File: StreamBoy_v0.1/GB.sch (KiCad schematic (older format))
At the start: 43 parts, among them J1 GB-CART, U2 LSF0204PWR, U3 LSF0204PWR

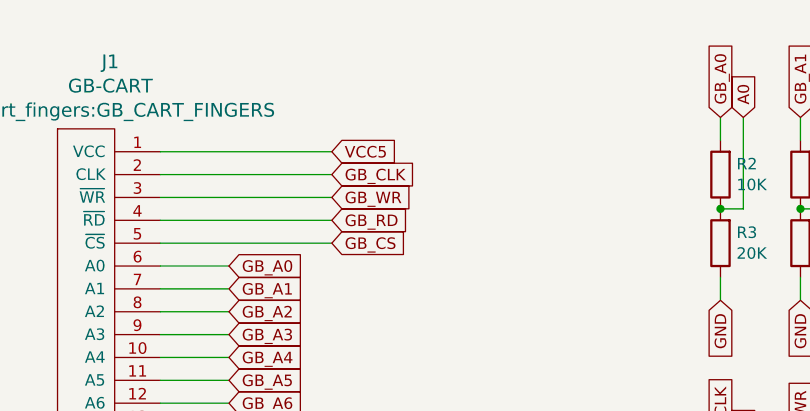
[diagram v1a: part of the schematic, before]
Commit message: Bunch of stuff
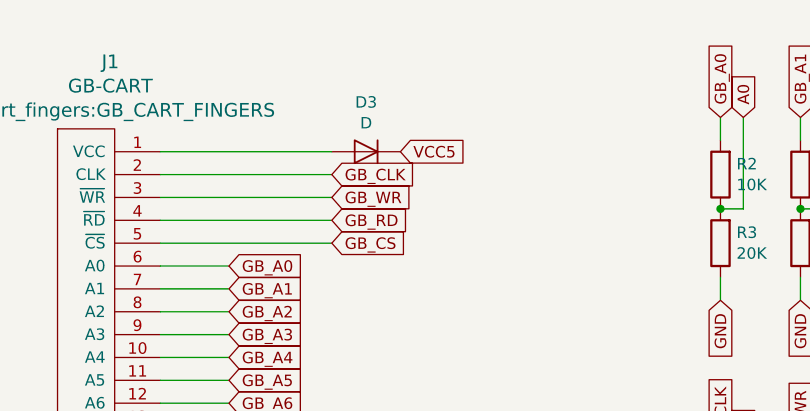
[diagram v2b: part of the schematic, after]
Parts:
- added D3: D, Diode_SMD:D_0805_2012Metric, symbol Device:D
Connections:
- net VCC5: now also D3.1 (K); no longer J1.1 (VCC)
- new net: D3.2 (A), J1.1 (VCC)
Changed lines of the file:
@@
 Text GLabel 3250 1550 2    50   Input ~ 0
 GB_WR
-Text GLabel 3250 1350 2    50   Input ~ 0
-VCC5
 Text GLabel 3250 1450 2    50   Input ~ 0
 GB_CLK
@@
 Text GLabel 3850 6050 0    50   Input ~ 0
 VCC3
+$Comp
+L Device:D D3
+U 1 1 5E09B24F
+P 3400 1350
+F 0 "D3" H 3400 1134 50  0000 C CNN
+F 1 "D" H 3400 1225 50  0000 C CNN
+F 2 "Diode_SMD:D_0805_2012Metric" H 3400 1350 50  0001 C CNN
+F 3 "~" H 3400 1350 50  0001 C CNN
+	1    3400 1350
+	-1   0    0    1
+$EndComp
+Text GLabel 3550 1350 2    50   Input ~ 0
+VCC5
 $EndSCHEMATC

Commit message: Power to the masses
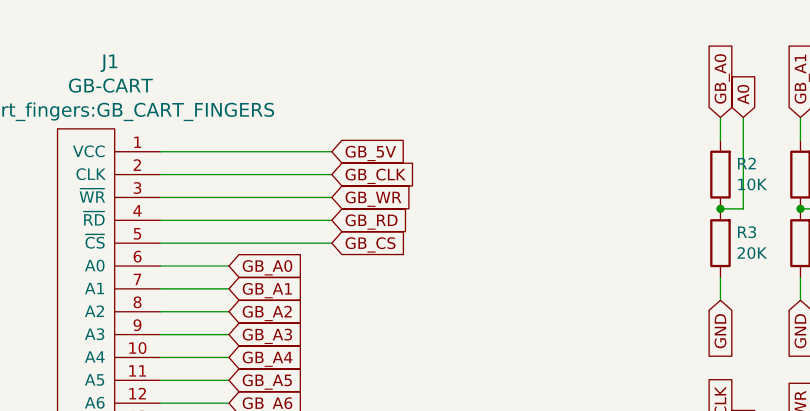
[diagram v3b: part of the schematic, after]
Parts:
- removed D3: D, Diode_SMD:D_0805_2012Metric, symbol Device:D
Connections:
- net GB_5V: now reaches J1.1 (VCC)
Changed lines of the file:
@@
 Text GLabel 3850 6050 0    50   Input ~ 0
 VCC3
-$Comp
-L Device:D D3
-U 1 1 5E09B24F
-P 3400 1350
-F 0 "D3" H 3400 1134 50  0000 C CNN
-F 1 "D" H 3400 1225 50  0000 C CNN
-F 2 "Diode_SMD:D_0805_2012Metric" H 3400 1350 50  0001 C CNN
-F 3 "~" H 3400 1350 50  0001 C CNN
-	1    3400 1350
-	-1   0    0    1
-$EndComp
-Text GLabel 3550 1350 2    50   Input ~ 0
-VCC5
+Text GLabel 3250 1350 2    50   Input ~ 0
+GB_5V
 $EndSCHEMATC

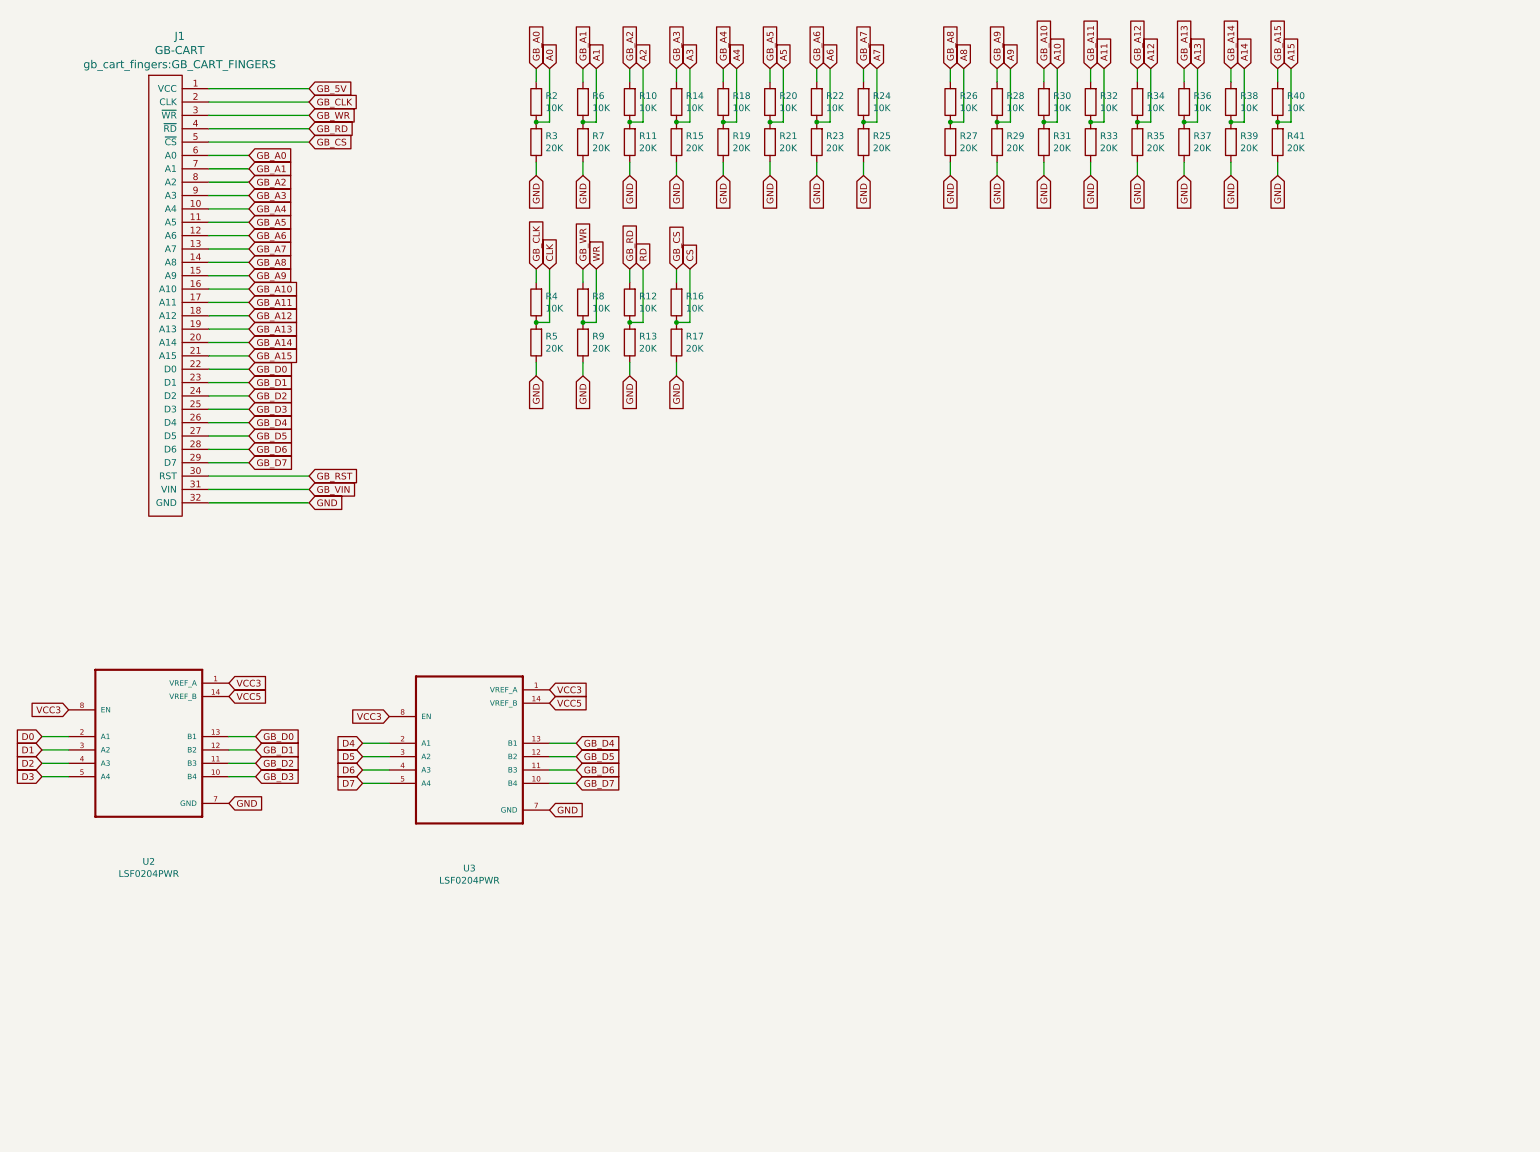
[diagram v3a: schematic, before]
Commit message: Temp
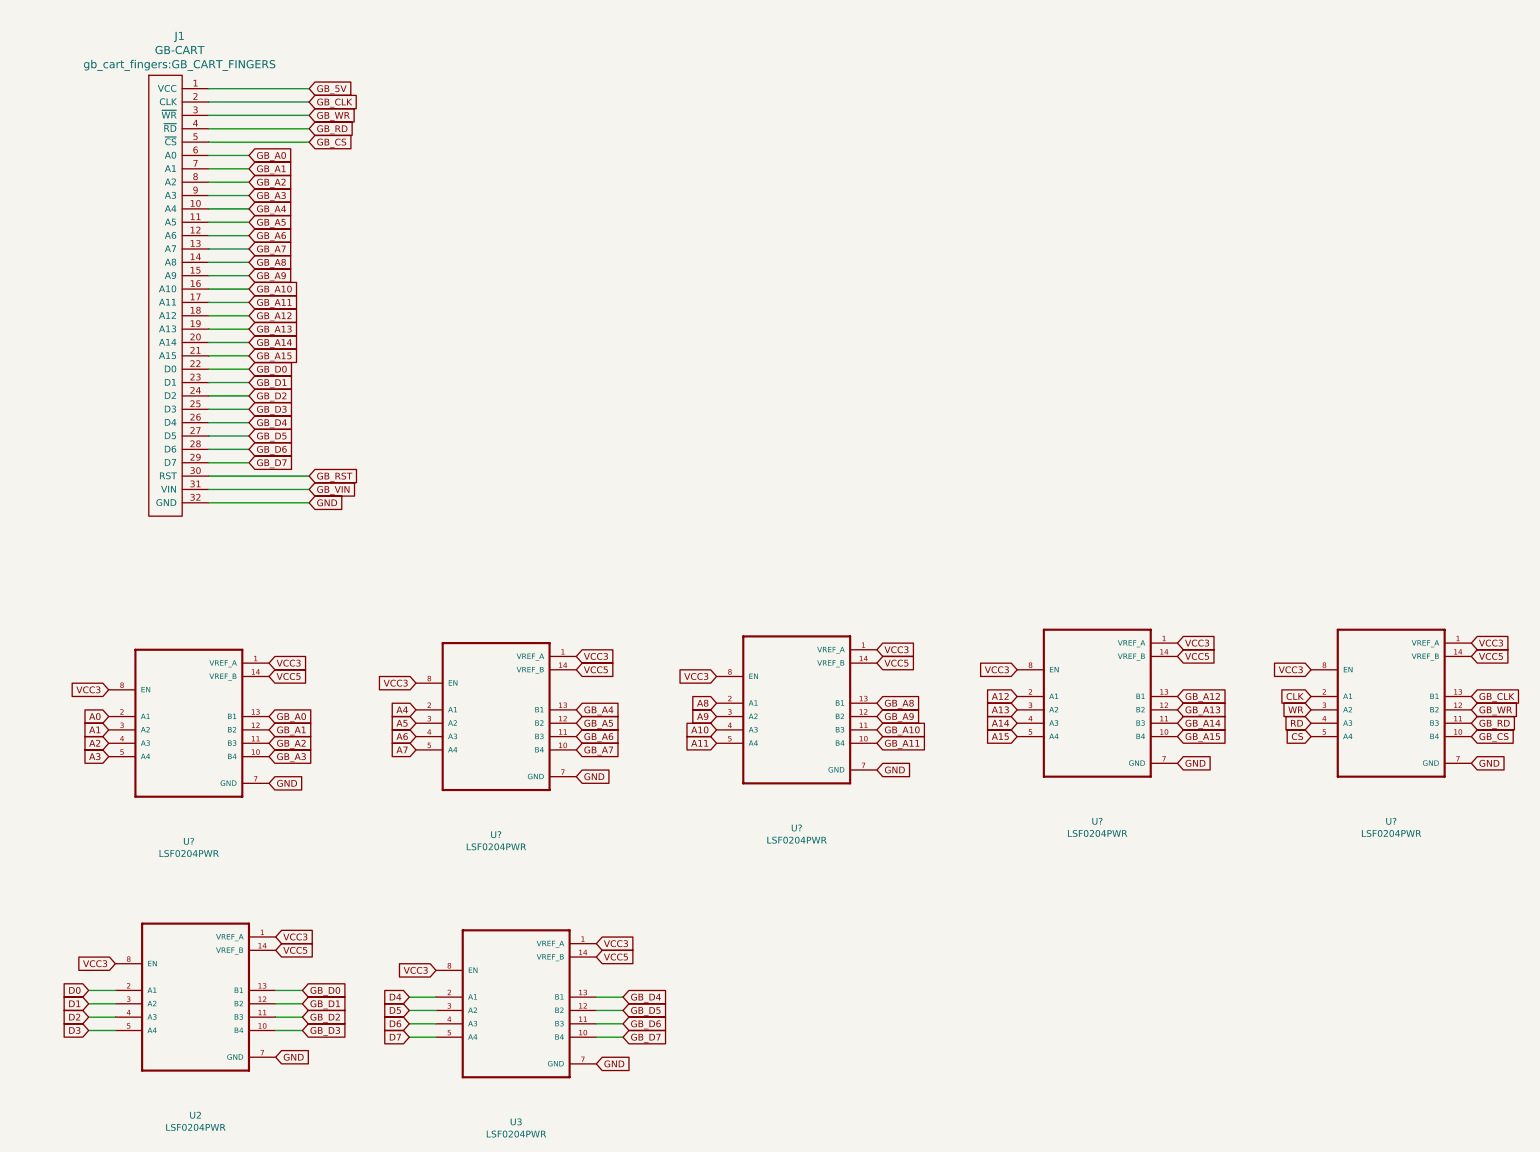
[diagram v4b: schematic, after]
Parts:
- removed R10, R12, R14, R16, R18, R2, R20, R22, R24, R26, R28, R30, R32, R34, R36, R38, R4, R40, R6, R8: 10K, Resistor_SMD:R_0805_2012Metric, symbol Device:R
- removed R11, R13, R15, R17, R19, R21, R23, R25, R27, R29, R3, R31, R33, R35, R37, R39, R41, R5, R7, R9: 20K, Resistor_SMD:R_0805_2012Metric, symbol Device:R
- added U? (x5): LSF0204PWR, LSF0204PWR:SOP65P640X120-14N, symbol LSF0204PWR:LSF0204PWR
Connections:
- net A0: now also U?.2 (A1)
- net A1: now also U?.3 (A2)
- net A10: now also U?.4 (A3)
- net A11: now also U?.5 (A4)
- net A12: now also U?.2 (A1)
- net A13: now also U?.3 (A2)
- net A14: now also U?.4 (A3)
- net A15: now also U?.5 (A4)
- net A2: now also U?.4 (A3)
- net A3: now also U?.5 (A4)
- net A4: now also U?.2 (A1)
- net A5: now also U?.3 (A2)
- net A6: now also U?.4 (A3)
- net A7: now also U?.5 (A4)
- net A8: now also U?.2 (A1)
- net A9: now also U?.3 (A2)
- net CLK: now also U?.2 (A1)
- net CS: now also U?.5 (A4)
- net GB_A0: now also U?.13 (B1)
- net GB_A1: now also U?.12 (B2)
- net GB_A10: now also U?.11 (B3)
- net GB_A11: now also U?.10 (B4)
- net GB_A12: now also U?.13 (B1)
- net GB_A13: now also U?.12 (B2)
- net GB_A14: now also U?.11 (B3)
- net GB_A15: now also U?.10 (B4)
- net GB_A2: now also U?.11 (B3)
- net GB_A3: now also U?.10 (B4)
- net GB_A4: now also U?.13 (B1)
- net GB_A5: now also U?.12 (B2)
- net GB_A6: now also U?.11 (B3)
- net GB_A7: now also U?.10 (B4)
- net GB_A8: now also U?.13 (B1)
- net GB_A9: now also U?.12 (B2)
- net GB_CLK: now also U?.13 (B1)
- net GB_CS: now also U?.10 (B4)
- net GB_RD: now also U?.11 (B3)
- net GB_WR: now also U?.12 (B2)
- net GND: now also U?.7 (GND), U?.7 (GND), U?.7 (GND), U?.7 (GND), U?.7 (GND)
- net RD: now also U?.4 (A3)
- net VCC3: now also U?.1 (VREF_A), U?.1 (VREF_A), U?.1 (VREF_A), U?.1 (VREF_A), U?.1 (VREF_A), U?.8 (EN), U?.8 (EN), U?.8 (EN), U?.8 (EN), U?.8 (EN)
- net VCC5: now also U?.14 (VREF_B), U?.14 (VREF_B), U?.14 (VREF_B), U?.14 (VREF_B), U?.14 (VREF_B)
- net WR: now also U?.3 (A2)
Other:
- moved on the sheet: U2, U3
